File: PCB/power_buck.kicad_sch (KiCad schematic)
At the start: 6 parts

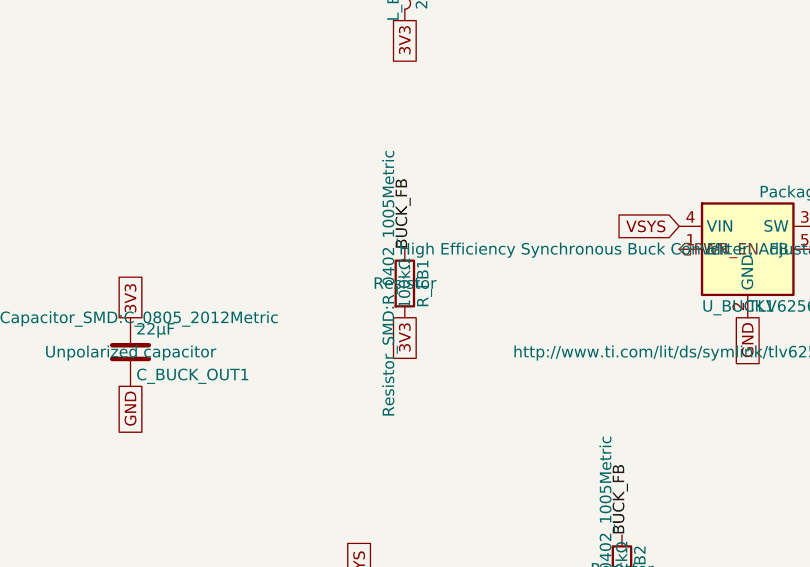
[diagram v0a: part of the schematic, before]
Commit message: task: first validation pass
This is the results post first kicad-happy run.
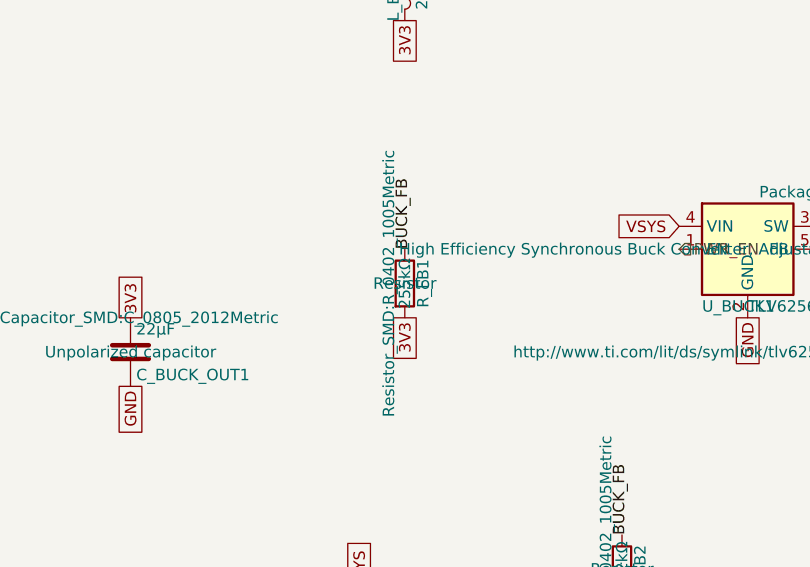
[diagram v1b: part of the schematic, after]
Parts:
- R_FB1: value 100kΩ -> 255kΩ
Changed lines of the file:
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@@
 			)
 		)
-		(property "Value" "100kΩ"
+		(property "Value" "255kΩ"
 			(at 144.78 101.6 90)
 			(show_name no)
